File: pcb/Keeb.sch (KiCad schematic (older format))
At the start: 39 parts, among them J1 TRRS_SJ1-42514, SW1 SW_RST, U1 ATMEGA32U4, U2 SN74HC138D‎, U3 SN74HC251, X1 XTAL_GND

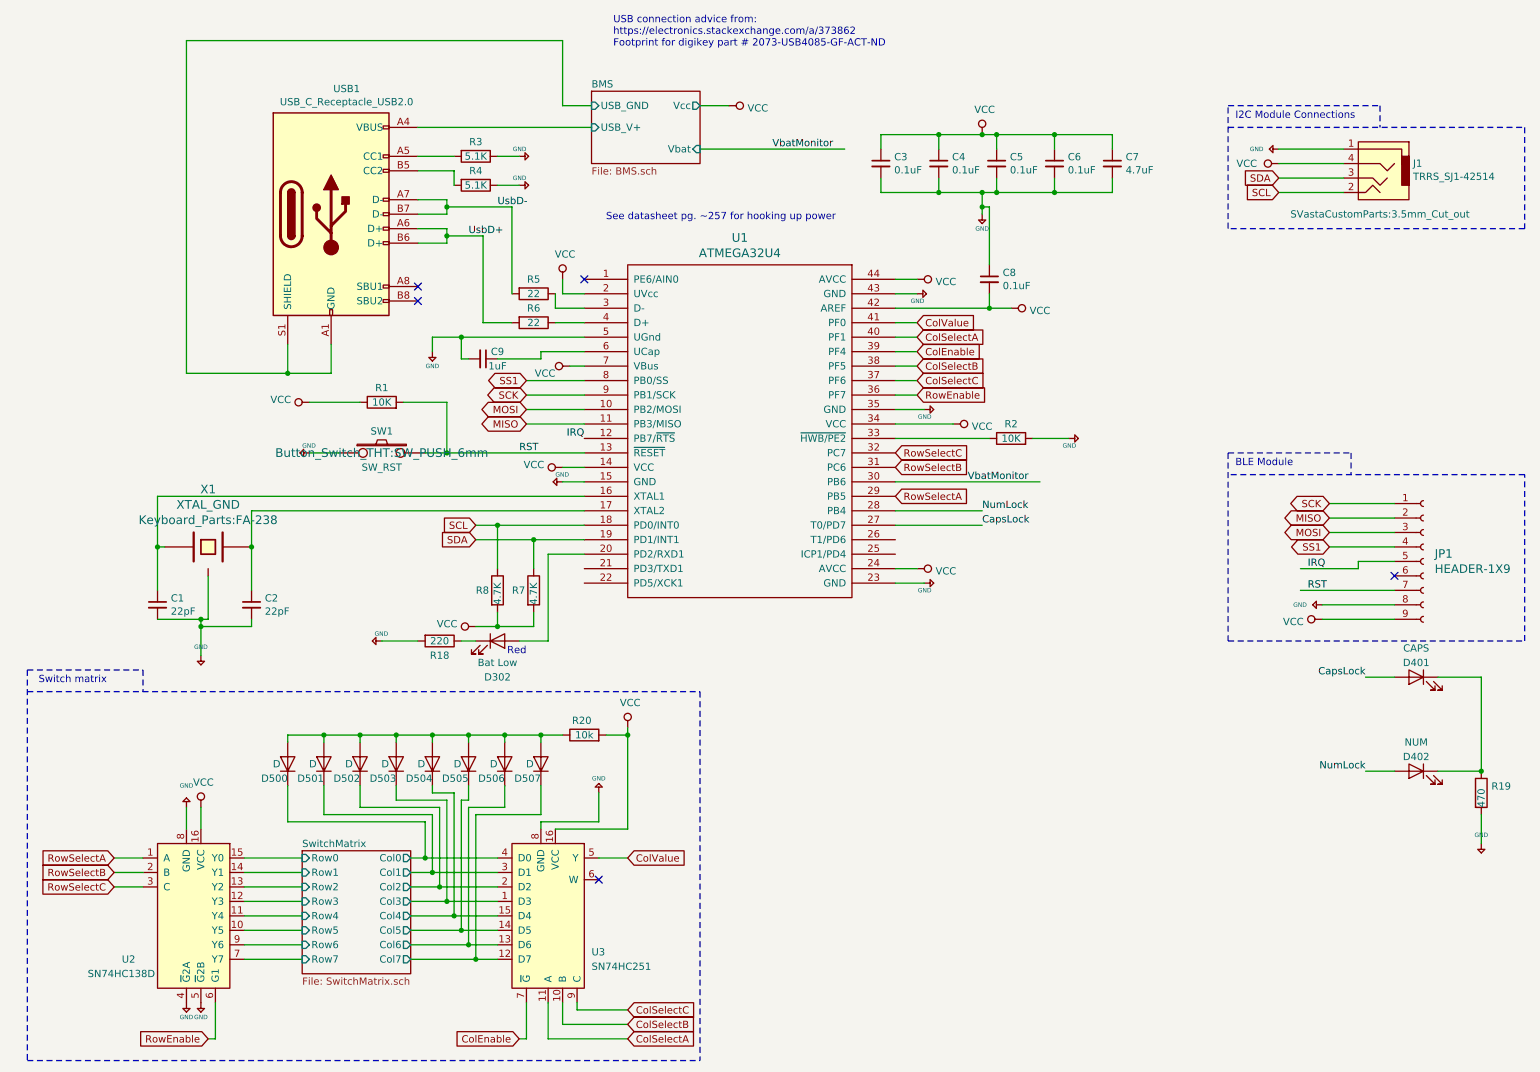
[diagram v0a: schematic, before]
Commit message: Layout & cad work for split pcb design
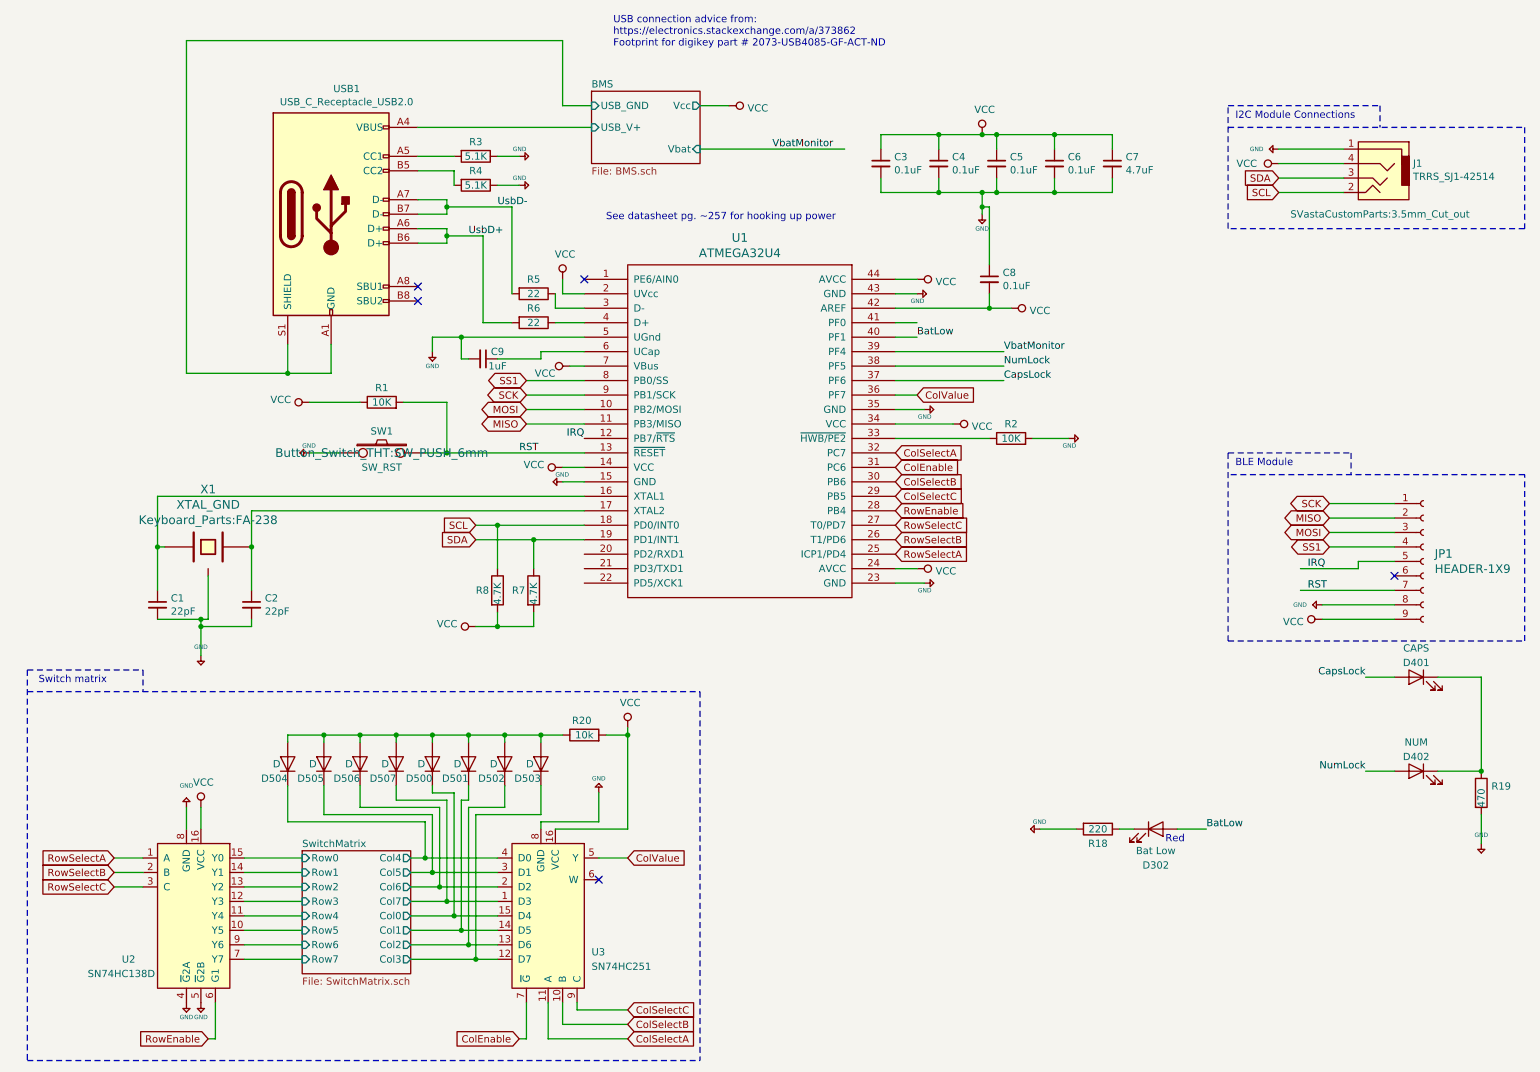
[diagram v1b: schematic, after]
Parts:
- renumbered D504 to D500, D505 to D501, D506 to D502, D507 to D503, D500 to D504, D501 to D505, D502 to D506, D503 to D507
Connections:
- net CapsLock: now also U1.37 (PF6); no longer U1.27 (T0/PD7)
- net ColEnable: now also U1.31 (PC6); no longer U1.39 (PF4)
- net ColSelectA: now also U1.32 (PC7); no longer U1.40 (PF1)
- net ColSelectB: now also U1.30 (PB6); no longer U1.38 (PF5)
- net ColSelectC: now also U1.29 (PB5); no longer U1.37 (PF6)
- net ColValue: now also U1.36 (PF7); no longer U1.41 (PF0)
- net NumLock: now also U1.38 (PF5); no longer U1.28 (PB4)
- net RowEnable: now also U1.28 (PB4); no longer U1.36 (PF7)
- net RowSelectA: now also U1.25 (ICP1/PD4); no longer U1.29 (PB5)
- net RowSelectB: now also U1.26 (T1/PD6); no longer U1.31 (PC6)
- net RowSelectC: now also U1.27 (T0/PD7); no longer U1.32 (PC7)
- net SwitchMatrix/Col0: now also D500.1 (K), U3.15 (D4); no longer D504.1 (K), U3.4 (D0)
- net SwitchMatrix/Col1: now also D501.1 (K), U3.14 (D5); no longer D505.1 (K), U3.3 (D1)
- net SwitchMatrix/Col2: now also D502.1 (K), U3.13 (D6); no longer D506.1 (K), U3.2 (D2)
- net SwitchMatrix/Col3: now also D503.1 (K), U3.12 (D7); no longer D507.1 (K), U3.1 (D3)
- net SwitchMatrix/Col4: now also D504.1 (K), U3.4 (D0); no longer D500.1 (K), U3.15 (D4)
- net SwitchMatrix/Col5: now also D505.1 (K), U3.3 (D1); no longer D501.1 (K), U3.14 (D5)
- net SwitchMatrix/Col6: now also D506.1 (K), U3.2 (D2); no longer D502.1 (K), U3.13 (D6)
- net SwitchMatrix/Col7: now also D507.1 (K), U3.1 (D3); no longer D503.1 (K), U3.12 (D7)
- net VbatMonitor: now also U1.39 (PF4); no longer U1.30 (PB6)
- net at U1.20 (PD2/RXD1): no longer D302.2 (A)
- new net BatLow: D302.2 (A), U1.40 (PF1)
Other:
- moved on the sheet: D302, R18
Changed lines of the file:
@@
 Text Label 9550 4500 0    50   ~ 0
 RST
-Text GLabel 6850 2650 2    50   Input ~ 0
-ColValue
 Text Label 9550 4350 0    50   ~ 0
 IRQ
@@
 Wire Wire Line
 	6850 3150 6700 3150
-Wire Wire Line
-	6700 3050 6850 3050
-Wire Wire Line
-	6850 2950 6700 2950
-Text GLabel 6850 3050 2    50   Input ~ 0
+Text GLabel 6700 3850 2    50   Input ~ 0
 ColSelectC
-Text GLabel 6850 2950 2    50   Input ~ 0
+Text GLabel 6700 3750 2    50   Input ~ 0
 ColSelectB
-Text GLabel 6850 2750 2    50   Input ~ 0
-ColSelectA
-Wire Wire Line
-	6700 2850 6850 2850
 Wire Wire Line
 	6850 2750 6700 2750
 Wire Wire Line
 	6700 2650 6850 2650
-Text GLabel 6700 3550 2    50   Input ~ 0
+Text GLabel 6700 4050 2    50   Input ~ 0
 RowSelectC
-Text GLabel 6700 3650 2    50   Input ~ 0
+Text GLabel 6700 4150 2    50   Input ~ 0
 RowSelectB
-Text GLabel 6700 3850 2    50   Input ~ 0
+Text GLabel 6700 4250 2    50   Input ~ 0
 RowSelectA
 Text GLabel 9700 4200 0    50   BiDi ~ 0
@@
 L Keyboard_Parts:GND #PWR0135
 U 1 1 5DA4D518
-P 3150 4850
-F 0 "#PWR0135" H 3150 4900 20  0001 C CNN
-F 1 "GND" V 3100 4800 30  0000 L CNN
-F 2 "" H 3150 4850 60  0000 C CNN
-F 3 "" H 3150 4850 60  0000 C CNN
-	1    3150 4850
+P 7700 6150
+F 0 "#PWR0135" H 7700 6200 20  0001 C CNN
+F 1 "GND" V 7650 6100 30  0000 L CNN
+F 2 "" H 7700 6150 60  0000 C CNN
+F 3 "" H 7700 6150 60  0000 C CNN
+	1    7700 6150
 	0    1    1    0
 $EndComp
@@
 Wire Wire Line
 	5350 1450 6350 1450
-Text Label 7200 3750 0    50   ~ 0
+Text Label 7450 2850 0    50   ~ 0
 VbatMonitor
-Wire Wire Line
-	6700 3750 7700 3750
 Text Label 3950 1850 0    50   ~ 0
 UsbD-
@@
 	4400 5500 4250 5500
 $Comp
-L Device:D D500
+L Device:D D504
 U 1 1 5E87864C
 P 2500 5700
-F 0 "D500" V 2400 5700 50  0000 L CNN
+F 0 "D504" V 2400 5700 50  0000 L CNN
 F 1 "D" V 2500 5750 50  0000 L CNN
 F 2 "SVastaCustomParts:D_MiniMELF_Handsoldering_Shorter_Pads" H 2500 5700 50  0001 C CNN
@@
 $EndComp
 $Comp
-L Device:D D501
+L Device:D D505
 U 1 1 5F0F89F1
 P 2750 5700
-F 0 "D501" V 2650 5700 50  0000 L CNN
+F 0 "D505" V 2650 5700 50  0000 L CNN
 F 1 "D" V 2750 5750 50  0000 L CNN
 F 2 "SVastaCustomParts:D_MiniMELF_Handsoldering_Shorter_Pads" H 2750 5700 50  0001 C CNN
@@
 $EndComp
 $Comp
-L Device:D D502
+L Device:D D506
 U 1 1 5F111C81
 P 3000 5700
-F 0 "D502" V 2900 5700 50  0000 L CNN
+F 0 "D506" V 2900 5700 50  0000 L CNN
 F 1 "D" V 3000 5750 50  0000 L CNN
 F 2 "SVastaCustomParts:D_MiniMELF_Handsoldering_Shorter_Pads" H 3000 5700 50  0001 C CNN
@@
 $EndComp
 $Comp
-L Device:D D503
+L Device:D D507
 U 1 1 5F12AF57
 P 3250 5700
-F 0 "D503" V 3150 5700 50  0000 L CNN
+F 0 "D507" V 3150 5700 50  0000 L CNN
 F 1 "D" V 3250 5750 50  0000 L CNN
 F 2 "SVastaCustomParts:D_MiniMELF_Handsoldering_Shorter_Pads" H 3250 5700 50  0001 C CNN
@@
 $EndComp
 $Comp
-L Device:D D504
+L Device:D D500
 U 1 1 5F144174
 P 3500 5700
-F 0 "D504" V 3400 5700 50  0000 L CNN
+F 0 "D500" V 3400 5700 50  0000 L CNN
 F 1 "D" V 3500 5750 50  0000 L CNN
 F 2 "SVastaCustomParts:D_MiniMELF_Handsoldering_Shorter_Pads" H 3500 5700 50  0001 C CNN
@@
 $EndComp
 $Comp
-L Device:D D505
+L Device:D D501
 U 1 1 5F15D38C
 P 3750 5700
-F 0 "D505" V 3650 5700 50  0000 L CNN
+F 0 "D501" V 3650 5700 50  0000 L CNN
 F 1 "D" V 3750 5750 50  0000 L CNN
 F 2 "SVastaCustomParts:D_MiniMELF_Handsoldering_Shorter_Pads" H 3750 5700 50  0001 C CNN
@@
 $EndComp
 $Comp
-L Device:D D506
+L Device:D D502
 U 1 1 5F176621
 P 4000 5700
-F 0 "D506" V 3900 5700 50  0000 L CNN
+F 0 "D502" V 3900 5700 50  0000 L CNN
 F 1 "D" V 4000 5750 50  0000 L CNN
 F 2 "SVastaCustomParts:D_MiniMELF_Handsoldering_Shorter_Pads" H 4000 5700 50  0001 C CNN
@@
 $EndComp
 $Comp
-L Device:D D507
+L Device:D D503
 U 1 1 5F18F99C
 P 4250 5700
-F 0 "D507" V 4150 5700 50  0000 L CNN
+F 0 "D503" V 4150 5700 50  0000 L CNN
 F 1 "D" V 4250 5750 50  0000 L CNN
 F 2 "SVastaCustomParts:D_MiniMELF_Handsoldering_Shorter_Pads" H 4250 5700 50  0001 C CNN
@@
 	0    -1   -1   0
 $EndComp
-Text GLabel 6850 3150 2    50   Input ~ 0
+Text GLabel 6700 3950 2    50   Input ~ 0
 RowEnable
-Text GLabel 6850 2850 2    50   Input ~ 0
+Text GLabel 6700 3650 2    50   Input ~ 0
 ColEnable
 Wire Wire Line
@@
 ColValue
 Wire Wire Line
-	3700 4850 3800 4850
+	8250 6150 8350 6150
 $Comp
 L Device:R R18
 U 1 1 5DACB6C1
-P 3550 4850
-F 0 "R18" V 3650 4850 50  0000 C CNN
-F 1 "220" V 3550 4850 50  0000 C CNN
-F 2 "Resistor_SMD:R_0805_2012Metric_Pad1.15x1.40mm_HandSolder" V 3480 4850 50  0001 C CNN
-F 3 "~" H 3550 4850 50  0001 C CNN
-	1    3550 4850
+P 8100 6150
+F 0 "R18" V 8200 6150 50  0000 C CNN
+F 1 "220" V 8100 6150 50  0000 C CNN
+F 2 "Resistor_SMD:R_0805_2012Metric_Pad1.15x1.40mm_HandSolder" V 8030 6150 50  0001 C CNN
+F 3 "~" H 8100 6150 50  0001 C CNN
+	1    8100 6150
 	0    1    1    0
 $EndComp
-Text Notes 4150 4950 2    50   ~ 0
+Text Notes 8700 6250 2    50   ~ 0
 Red
 Wire Wire Line
-	3400 4850 3150 4850
+	7950 6150 7700 6150
 $Comp
 L Device:LED D?
 U 1 1 5DA415D4
-P 3950 4850
+P 8500 6150
 AR Path="/5DF457A9/5DA415D4" Ref="D?"  Part="1"
 AR Path="/5DA415D4" Ref="D302"  Part="1"
-F 0 "D302" H 3950 4600 50  0000 C CNN
-F 1 "Bat Low" H 3950 4700 50  0000 C CNN
-F 2 "LED_SMD:LED_0805_2012Metric_Pad1.15x1.40mm_HandSolder" H 3950 4850 50  0001 C CNN
-F 3 "~" H 3950 4850 50  0001 C CNN
-	1    3950 4850
-	1    0    0    -1
-$EndComp
-Wire Wire Line
-	4550 4250 4300 4250
-Wire Wire Line
-	4300 4250 4300 4850
-Wire Wire Line
-	4300 4850 4100 4850
-Text Label 7300 4050 0    50   ~ 0
+F 0 "D302" H 8500 5900 50  0000 C CNN
+F 1 "Bat Low" H 8500 6000 50  0000 C CNN
+F 2 "LED_SMD:LED_0805_2012Metric_Pad1.15x1.40mm_HandSolder" H 8500 6150 50  0001 C CNN
+F 3 "~" H 8500 6150 50  0001 C CNN
+	1    8500 6150
+	1    0    0    -1
+$EndComp
+Wire Wire Line
+	8850 6150 8650 6150
+Text Label 7450 3050 0    50   ~ 0
 CapsLock
-Text Label 7300 3950 0    50   ~ 0
+Text Label 7450 2950 0    50   ~ 0
 NumLock
 Wire Wire Line
@@
 Wire Notes Line
 	9000 2000 9000 1150
-Wire Wire Line
-	6700 3950 7300 3950
-Wire Wire Line
-	7300 4050 6700 4050
+Text GLabel 6700 3550 2    50   Input ~ 0
+ColSelectA
+Text GLabel 6850 3150 2    50   Input ~ 0
+ColValue
+Wire Wire Line
+	6700 3050 7450 3050
+Wire Wire Line
+	6700 2950 7450 2950
+Wire Wire Line
+	6700 2850 7450 2850
+Text Label 8850 6150 0    50   ~ 0
+BatLow
+Text Label 6850 2750 0    50   ~ 0
+BatLow
 $Sheet
 S 2600 6300 750  850
@@
 F5 "Row5" I L 2600 6850 50
 F6 "Row4" I L 2600 6750 50
-F7 "Col7" O R 3350 7050 50
+F7 "Col7" O R 3350 6650 50
 F8 "Row1" I L 2600 6450 50
 F9 "Row2" I L 2600 6550 50
 F10 "Row3" I L 2600 6650 50
-F11 "Col0" O R 3350 6350 50
-F12 "Col1" O R 3350 6450 50
-F13 "Col2" O R 3350 6550 50
-F14 "Col3" O R 3350 6650 50
-F15 "Col4" O R 3350 6750 50
-F16 "Col5" O R 3350 6850 50
-F17 "Col6" O R 3350 6950 50
+F11 "Col0" O R 3350 6750 50
+F12 "Col1" O R 3350 6850 50
+F13 "Col2" O R 3350 6950 50
+F14 "Col3" O R 3350 7050 50
+F15 "Col4" O R 3350 6350 50
+F16 "Col5" O R 3350 6450 50
+F17 "Col6" O R 3350 6550 50
 $EndSheet
 $EndSCHEMATC
